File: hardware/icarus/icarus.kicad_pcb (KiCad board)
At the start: 4 copper layers, 41.3 x 36.8 mm, 34 parts, among them J1 USB_B_Micro, J2 SWD, SW1 RST, SW2 BOOT, U1 STM32F302C8Tx, U2 AMS1117-3.3, U3 MPU-6050, U4 BMP388, U5 ICARUS, Y1 12MHz

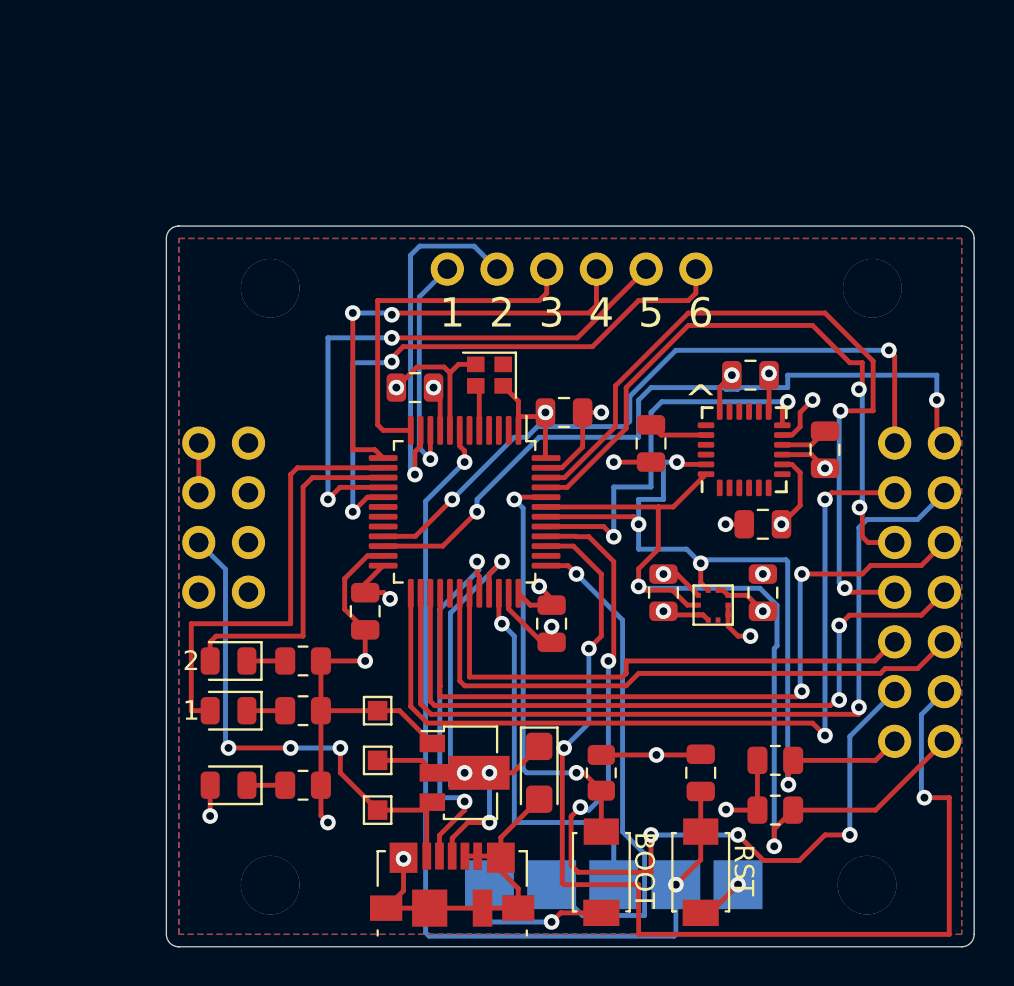
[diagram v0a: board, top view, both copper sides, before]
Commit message: Rev C
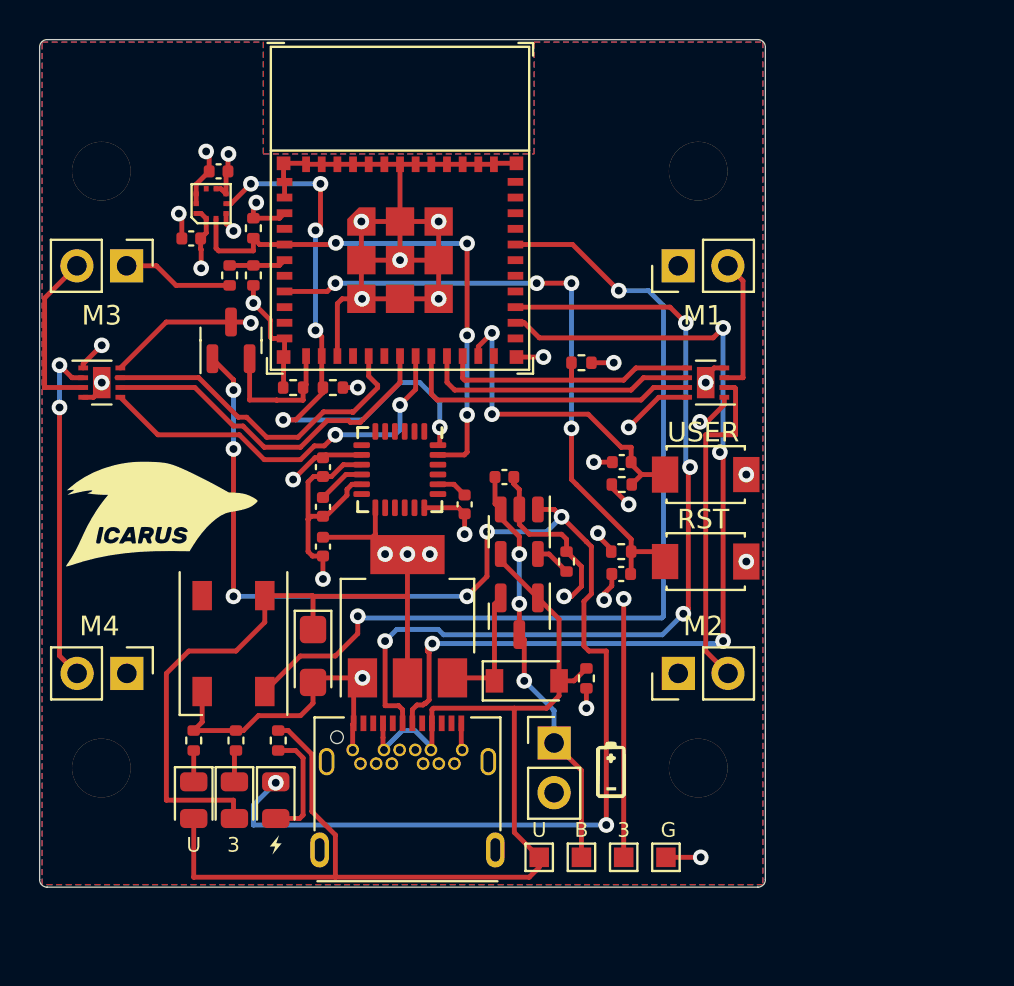
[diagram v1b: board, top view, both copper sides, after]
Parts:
- removed C11, C12: 100nF, Capacitor_SMD:C_0805_2012Metric
- removed J2: SWD, custom-breakout:SWD-bcu
- removed Y1: 12MHz, Crystal:Crystal_SMD_2016-4Pin_2.0x1.6mm
- added D4: STAT, LED_SMD:LED_WS2812B_PLCC4_5.0x5.0mm_P3.2mm, F.Cu at (140.6, 80.4)
- added D5: CHR, LED_SMD:LED_0805_2012Metric, F.Cu at (142.7, 88.4)
- added G***: LOGO, symbols:battery2_3, F.Cu at (159.9, 86.9)
- added G***: LOGO, icarus:icarus-logo, F.Cu at (136.9, 73.8)
- added G***: LOGO, symbols:charge_1x1, F.Cu at (142.7, 90.7)
- added G***: LOGO, symbols:radio1, B.Cu at (149.1, 52.6)
- added M1: RTR1, Connector_PinHeader_2.54mm:PinHeader_1x02_P2.54mm_Vertical, F.Cu at (163.3, 61.1)
- added M2: RTR2, Connector_PinHeader_2.54mm:PinHeader_1x02_P2.54mm_Vertical, F.Cu at (163.3, 81.9)
- added M3: RTR3, Connector_PinHeader_2.54mm:PinHeader_1x02_P2.54mm_Vertical, F.Cu at (135.1, 61.1)
- added M4: RTR4, Connector_PinHeader_2.54mm:PinHeader_1x02_P2.54mm_Vertical, F.Cu at (135.1, 81.9)
- added P1: USB_C_Plug_USB2.0, USB-C-Connectors:TYPE-C-31-M-04, F.Cu at (149.5, 89.5)
- added Q1: DMG2305, Package_TO_SOT_SMD:SOT-23, F.Cu at (155.2, 79.0)
- added Q2: 2N7002, Package_TO_SOT_SMD:SOT-23, F.Cu at (140.5, 64.9)
- added R1: 100k, Resistor_SMD:R_0402_1005Metric, F.Cu at (158.6, 82.2)
- added R10: 1k, Resistor_SMD:R_0402_1005Metric, F.Cu at (142.9, 85.3)
- added R11: 10k, Resistor_SMD:R_0402_1005Metric, F.Cu at (160.4, 75.7)
- added R12: 10k, Resistor_SMD:R_0402_1005Metric, F.Cu at (160.4, 72.3)
- added R13: 10k, Resistor_SMD:R_0402_1005Metric, F.Cu at (158.4, 66.0)
- added R8: 4.7k, Resistor_SMD:R_0402_1005Metric, F.Cu at (157.6, 76.2)
- added R9: 100k, Resistor_SMD:R_0402_1005Metric, F.Cu at (143.6, 67.3)
- added REF**: mounting_holes_30.5mm, drone:mounting_holes_30.5mm, F.Cu at (149.1, 71.5)
- added TP4: GND, TestPoint:TestPoint_Pad_1.0x1.0mm, F.Cu at (162.7, 91.3)
- added U6: BMP388, sensors:BMP388, F.Cu at (139.4, 57.9)
- added U7: ESP32-C3-MINI-1, Espressif:ESP32-C3-MINI-1, F.Cu at (149.1, 60.8)
- C10: value 10nF -> 100nF; footprint Capacitor_SMD:C_0805_2012Metric -> Capacitor_SMD:C_0402_1005Metric
- C2, C5, C7, C8: footprint Capacitor_SMD:C_0805_2012Metric -> Capacitor_SMD:C_0402_1005Metric
- C3: value 4.7uF -> 2.2nF; footprint Capacitor_SMD:C_0805_2012Metric -> Capacitor_SMD:C_0402_1005Metric
- C4: value 100nF -> 10nF; footprint Capacitor_SMD:C_0805_2012Metric -> Capacitor_SMD:C_0402_1005Metric
- C6: value 100nF -> 4.7uF; footprint Capacitor_SMD:C_0805_2012Metric -> Capacitor_SMD:C_0402_1005Metric
- C9: value 2.2nF -> 100nF; footprint Capacitor_SMD:C_0805_2012Metric -> Capacitor_SMD:C_0402_1005Metric
- D1: value PWR -> B5819W; footprint LED_SMD:LED_0805_2012Metric -> Diode_SMD:D_SOD-123
- D2: value STAT1 -> 5V
- D3: value STAT2 -> 3V3
- J1: value USB_B_Micro -> BAT; footprint Connector_USB:USB_Micro-B_Molex_47346-0001 -> Connector_PinHeader_2.54mm:PinHeader_1x02_P2.54mm_Vertical
- R2, R7: value 200 -> 10k; footprint Resistor_SMD:R_0805_2012Metric -> Resistor_SMD:R_0402_1005Metric
- R3: footprint Resistor_SMD:R_0805_2012Metric -> Resistor_SMD:R_0402_1005Metric
- R4: value 10k -> 1k; footprint Resistor_SMD:R_0805_2012Metric -> Resistor_SMD:R_0402_1005Metric
- R5: value 10k -> 560; footprint Resistor_SMD:R_0805_2012Metric -> Resistor_SMD:R_0402_1005Metric
- R6: value 200 -> 6.8k; footprint Resistor_SMD:R_0805_2012Metric -> Resistor_SMD:R_0402_1005Metric
- SW1: value RST -> USER
- SW2: value BOOT -> RST
- TP1: value 3V3 -> VBUS
- TP2: value 5V -> BATT
- U1: value STM32F302C8Tx -> AMS1117-3.3; footprint Package_QFP:LQFP-48_7x7mm_P0.5mm -> Package_TO_SOT_SMD:SOT-223-3_TabPin2
- U2: value AMS1117-3.3 -> DRV8837; footprint Package_TO_SOT_SMD:SOT-89-3 -> Package_SON:WSON-8-1EP_2x2mm_P0.5mm_EP0.9x1.6mm
- U3: value MPU-6050 -> DRV8837; footprint Sensor_Motion:InvenSense_QFN-24_4x4mm_P0.5mm -> Package_SON:WSON-8-1EP_2x2mm_P0.5mm_EP0.9x1.6mm
- U4: value BMP388 -> MPU-6050; footprint sensors:BMP388 -> Sensor_Motion:InvenSense_QFN-24_4x4mm_P0.5mm
- U5: value ICARUS -> MCP73831-2-OT; footprint icarus:icarus-shield -> Package_TO_SOT_SMD:SOT-23-5
- moved R3 39.9 mm to (141.6, 59.2), turned to 90 degrees
- moved C8 34.1 mm to (139.8, 56.3), turned to 180 degrees
- moved R4 29.7 mm to (138.6, 85.3), turned to 90 degrees
- moved U2 27.2 mm to (133.9, 67.1)
- moved C2 22.9 mm to (145.2, 73.4), turned to -90 degrees
- moved R6 22.6 mm to (140.4, 61.6), turned to 90 degrees
- moved C4 22.5 mm to (145.2, 75.4)
- moved R2 20.4 mm to (145.7, 67.3)
- moved SW1 20.3 mm to (164.7, 71.8), turned to 180 degrees
- moved R7 19.9 mm to (141.6, 61.6), turned to -90 degrees
- moved R5 18.7 mm to (140.7, 85.3)
- moved U4 17.4 mm to (149.1, 71.5), turned to -90 degrees
- moved SW2 16.7 mm to (164.7, 76.2), turned to 0 degrees
- moved D1 16.1 mm to (155.6, 82.3), turned to 0 degrees
- moved U5 14.9 mm to (155.2, 74.7), turned to -90 degrees
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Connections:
- C10 pad 1: GND -> /user_btn
- C10 pad 2: +3V3 -> GND
- C2 pad 1: +3V3 -> Net-(C2-Pad1)
- C3 pad 1: +3V3 -> Net-(C3-Pad1)
- C4 pad 1: /nreset -> GND
- C4 pad 2: GND -> +3V3
- C5 pad 1: +3V3 -> GND
- C5 pad 2: GND -> +3V3
- C6 pad 1: +3V3 -> +BATT
- C8 pad 1: Net-(C8-Pad1) -> +3V3
- C9 pad 1: Net-(C9-Pad1) -> /nreset
- D1 pad 2: +3V3 -> VBUS
- D2 pad 2: /led1 -> VBUS
- D3 pad 2: /led2 -> +3V3
- J1 pad 1: VBUS -> +BATT
- J1 pad 2: /usb_fs_dm -> GND
- R2 pad 1: Net-(D1-Pad1) -> /sda
- R2 pad 2: GND -> +3V3
- R3 pad 1: +3V3 -> /scl
- R3 pad 2: /sda -> +3V3
- R4 pad 1: +3V3 -> Net-(D2-Pad1)
- R4 pad 2: /scl -> GND
- R5 pad 1: /boot0 -> Net-(D3-Pad1)
- R6 pad 1: Net-(D2-Pad1) -> +BATT
- R6 pad 2: GND -> Net-(R6-Pad2)
- R7 pad 1: Net-(D3-Pad1) -> Net-(R6-Pad2)
- SW1 pad 1: /nreset -> GND
- SW1 pad 2: GND -> /user_btn
- SW2 pad 1: /boot0 -> /nreset
- SW2 pad 2: +3V3 -> GND
- TP1 pad 1: +3V3 -> VBUS
- TP2 pad 1: VBUS -> +BATT
- TP3 pad 1: GND -> +3V3
- U1 pad 1: +3V3 -> GND
- U1 pad 2: unconnected-(U1-Pad2) -> +3V3
- U1 pad 3: unconnected-(U1-Pad3) -> Net-(D1-Pad1)
- U2 pad 1: GND -> +BATT
- U2 pad 2: +3V3 -> Net-(M4-Pad2)
- U2 pad 3: VBUS -> Net-(M3-Pad2)
- U3 pad 1: unconnected-(U3-Pad1) -> +BATT
- U3 pad 2: (no net) -> Net-(M2-Pad2)
- U3 pad 3: (no net) -> Net-(M1-Pad2)
- U3 pad 4: (no net) -> GND
- U3 pad 5: (no net) -> /rtrctl1
- U3 pad 6: unconnected-(U3-Pad6) -> /rtrctl2
- U3 pad 7: unconnected-(U3-Pad7) -> Net-(U3-Pad7)
- U4 pad 1: +3V3 -> unconnected-(U4-Pad1)
- U4 pad 10: +3V3 -> Net-(C2-Pad1)
- U4 pad 2: /scl -> (no net)
- U4 pad 3: GND -> (no net)
- U4 pad 4: /sda -> (no net)
- U4 pad 5: +3V3 -> (no net)
- U4 pad 6: +3V3 -> unconnected-(U4-Pad6)
- U4 pad 8: GND -> +3V3
- U5 pad 1: VDC -> Net-(D5-Pad1)
- U5 pad 3: VDC -> +BATT
- U5 pad 4: GND -> VBUS
- U5 pad 5: VBUS -> Net-(R8-Pad1)
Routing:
- net Net-(D5-Pad1): track 0.00 -> 71.9 mm, vias 0 -> 8
- net /usart2_tx: track 56.6 -> 0.00 mm, vias 3 -> 0
- net Net-(D4-Pad4): track 0.00 -> 47.3 mm, vias 0 -> 2
- net /usb_dm: track 0.00 -> 47.2 mm, vias 0 -> 4
- net /usart2_rx: track 46.7 -> 0.00 mm, vias 5 -> 0
- net /usb_dp: track 0.00 -> 45.2 mm, vias 0 -> 4
- net /gpio3: track 43.3 -> 0.00 mm, vias 2 -> 0
- net /sck: track 43.0 -> 0.00 mm, vias 1 -> 0
- net /can_tx: track 38.6 -> 0.00 mm, vias 2 -> 0
- net /mosi: track 38.0 -> 0.00 mm, vias 2 -> 0
- net /gpio2: track 37.5 -> 0.00 mm, vias 2 -> 0
- net /miso: track 36.6 -> 0.00 mm, vias 2 -> 0
- net VBUS: track 26.6 -> 62.3 mm, vias 3 -> 0
- net /gpio1: track 35.4 -> 0.00 mm, vias 2 -> 0
- net /can_rx: track 32.6 -> 0.00 mm, vias 2 -> 0
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- added copper zone on In1.Cu, net +BATT
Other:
- board size 41.3 x 36.8 mm -> 37.1 x 43.3 mm
- board text added: "B"
- board text added: "G"
- board text added: "RST"
- board text added: "U"
- board text added: "USER"
- board text added: "icarus :: Rev C nnarain"
- board text removed: "1"
- board text removed: "2"
- board text removed: "3V3"
- board text removed: "4"
- board text removed: "5"
- board text removed: "6"
- board text removed: "GND"
- board text removed: "NRST"
- board text removed: "SWCLK"
- board text removed: "SWDIO"
- board text removed: "^"
- board text removed: "icarus :: Rev B nnarain"
